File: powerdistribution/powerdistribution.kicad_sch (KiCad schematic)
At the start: 11 parts, among them J1 Conn_01x02_Socket, J2 Conn_01x02_Socket, J3 Conn_01x02_Socket, J4 Screw_Terminal_01x02, J5 Screw_Terminal_01x02, J6 Conn_01x10_Socket, J7 Conn_01x10_Socket, SW1 RA1H1C112R, SW2 RA1H1C112R, U1 BQ7790512PW

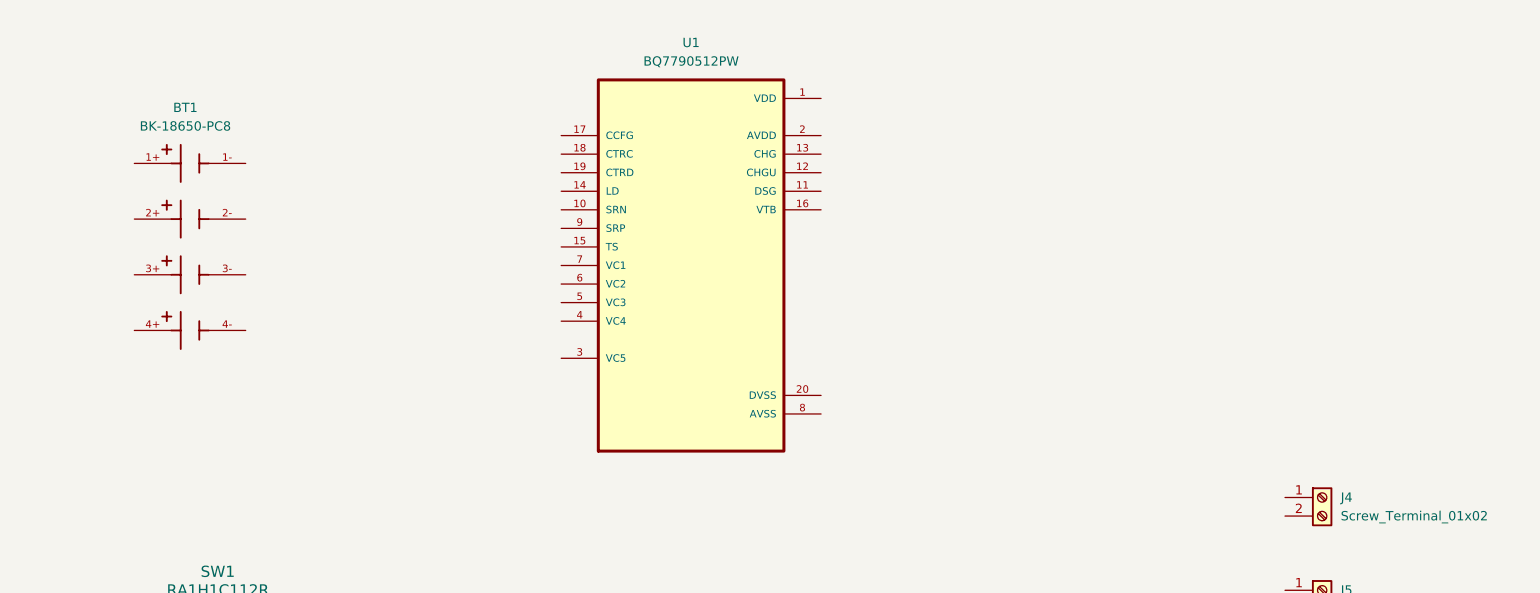
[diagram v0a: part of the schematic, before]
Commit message: BMS draft
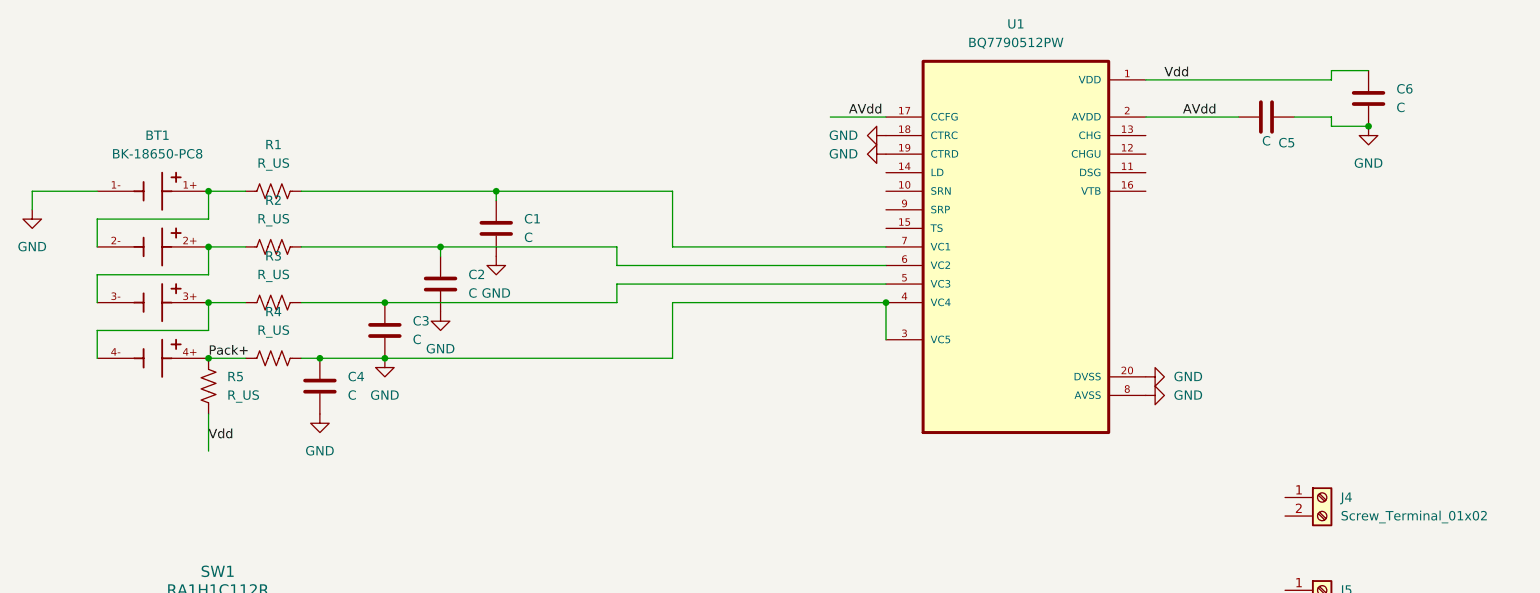
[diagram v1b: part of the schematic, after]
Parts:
- added C1, C2, C3, C4, C5, C6: C, symbol Device:C
- added R1, R2, R3, R4, R5: R_US, symbol Device:R_US
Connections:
- net Vdd: now reaches U1.1 (VDD)
- net Vdd: now also C6.2, R5.2
- net AVdd: now reaches U1.17 (CCFG)
- net AVdd: now also U1.2 (AVDD), C5.1
- net GND: now reaches U1.18 (CTRC)
- net GND: now also BT1.1-, U1.19 (CTRD), U1.20 (DVSS), U1.3 (VC5), U1.4 (VC4), U1.8 (AVSS), C1.2, C2.2, C3.2, C4.1, C4.2, C5.2, C6.1, R4.2
- net at U1.5 (VC3): now also C3.1, R3.2
- net at U1.6 (VC2): now also C2.1, R2.2
- net at U1.7 (VC1): now also C1.1, R1.2
- net at BT1.1+: now also BT1.2-, R1.1
- net at BT1.2+: now also BT1.3-, R2.1
- net at BT1.3+: now also BT1.4-, R3.1
- net Pack+: now reaches BT1.4+
- net Pack+: now also R4.1, R5.1
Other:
- moved on the sheet: BT1, U1

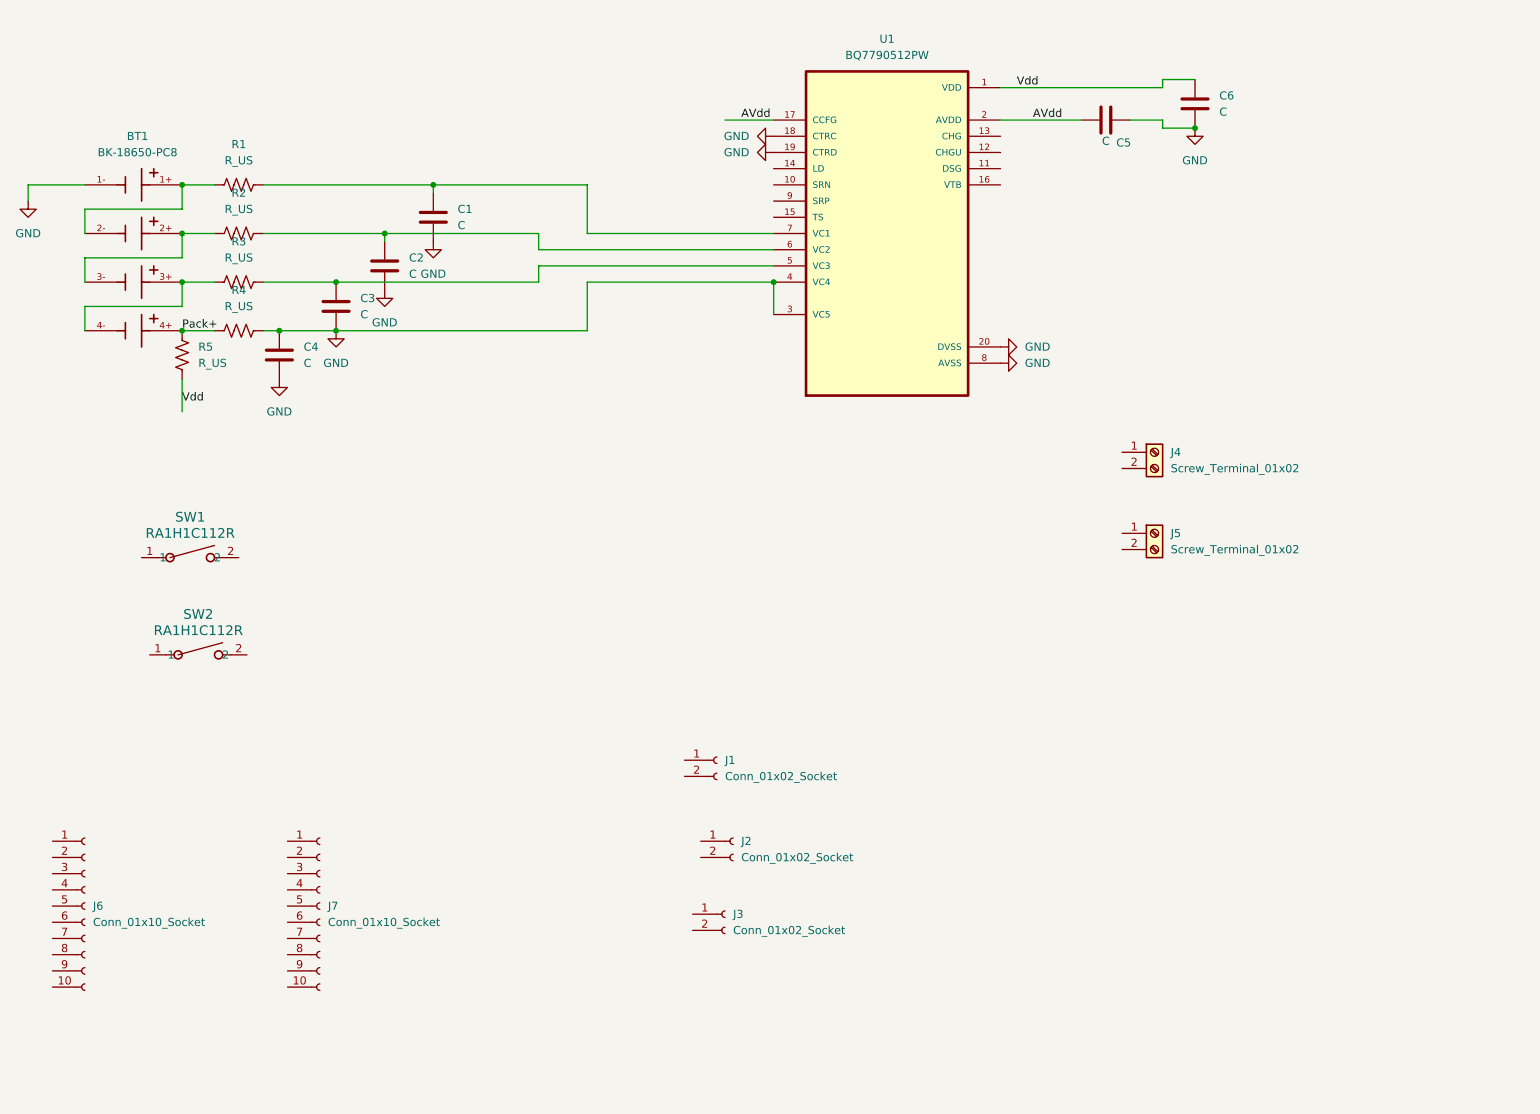
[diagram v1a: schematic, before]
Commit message: pwr draft
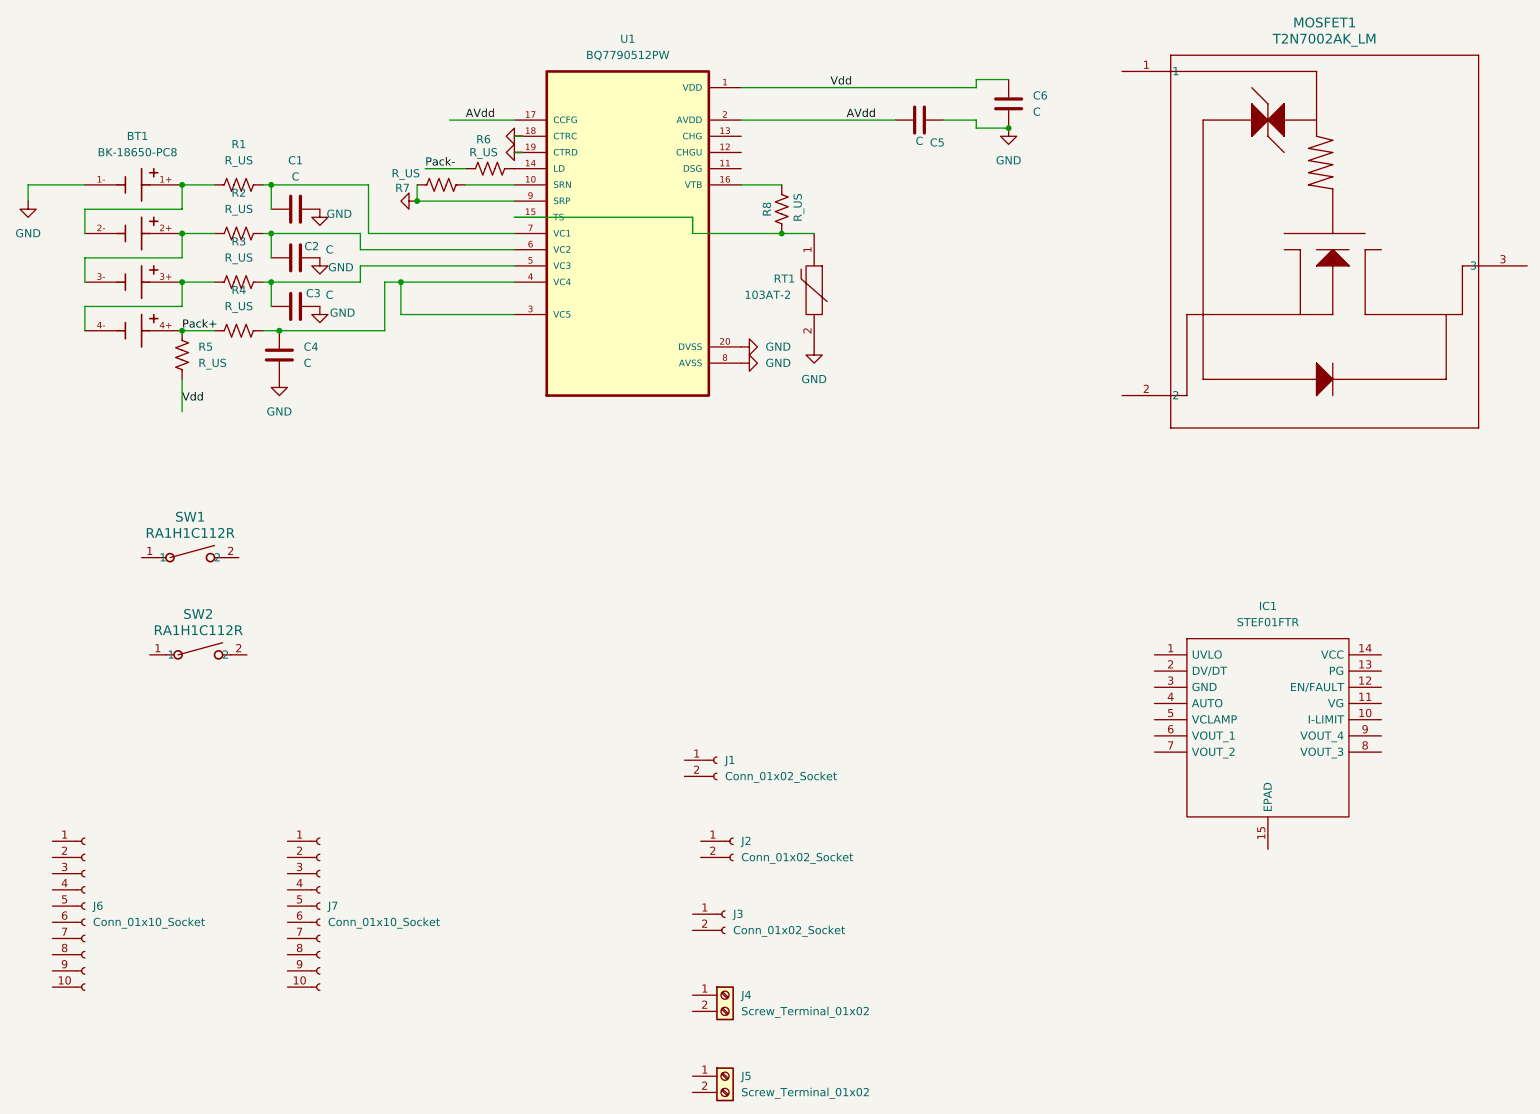
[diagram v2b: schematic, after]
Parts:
- added IC1: STEF01FTR, SOP65P640X120-15N, symbol HPRsymbols:STEF01FTR
- added MOSFET1: T2N7002AK_LM, SOT23_TOS, symbol HPRsymbols:T2N7002AK_LM
- added R6, R7, R8: R_US, symbol Device:R_US
- added RT1: 103AT-2, 103AT2, symbol HPRsymbols:103AT-2
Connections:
- net GND: now also U1.9 (SRP), R7.1, RT1.2; no longer C4.1, R4.2, U1.3 (VC5), U1.4 (VC4)
- net at U1.10 (SRN): now also R7.2
- net at U1.14 (LD): now also R6.2
- net at U1.15 (TS): now also R8.1, RT1.1
- net at U1.16 (VTB): now also R8.2
- new net: C4.1, R4.2, U1.3 (VC5), U1.4 (VC4)
- new net Pack-: R6.1
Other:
- moved on the sheet: C1, C2, C3, C5, C6, J4, J5, U1
